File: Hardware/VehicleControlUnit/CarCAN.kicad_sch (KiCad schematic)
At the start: 9 parts, among them IC2 TCAN3413DR

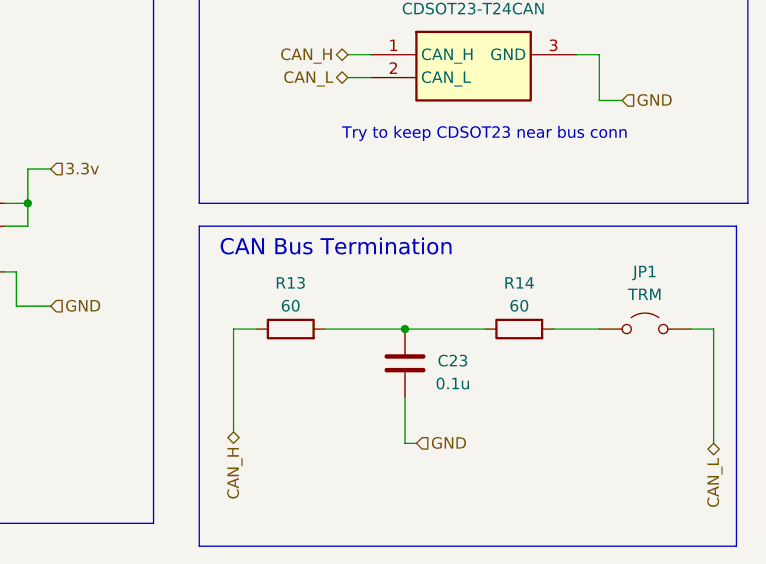
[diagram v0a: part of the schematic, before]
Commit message: 70% tracing done
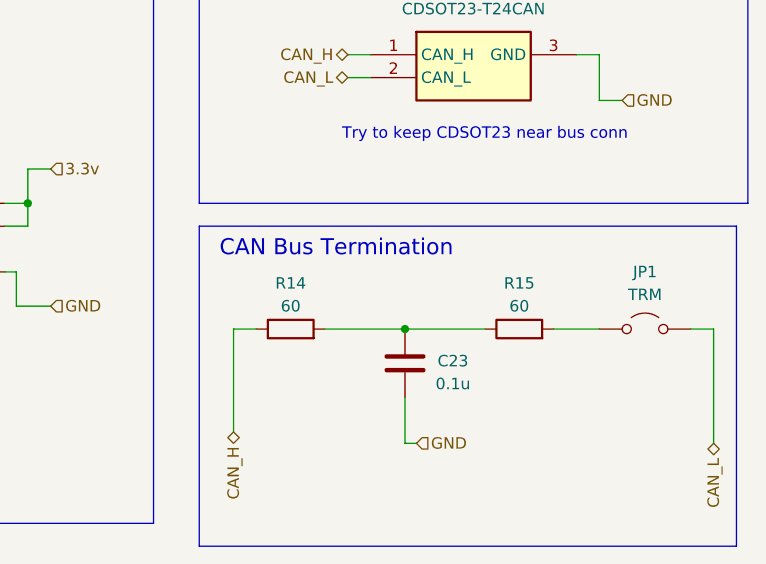
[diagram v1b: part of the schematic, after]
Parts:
- renumbered R13 to R14, R14 to R15
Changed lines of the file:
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@@
 		(in_pos_files yes)
 		(dnp no)
-		(property "Reference" "R14"
+		(property "Reference" "R15"
 			(at 201.93 80.01 90)
 			(show_name no)
@@
 			(project "VehicleControlUnit"
 				(path "/e864fac9-3897-46c9-9101-6d5488c6cd3a/252635d1-b56c-4964-8f6e-39efe20521e2"
-					(reference "R14")
+					(reference "R15")
 					(unit 1)
 				)
@@
 		(in_pos_files yes)
 		(dnp no)
-		(property "Reference" "R13"
+		(property "Reference" "R14"
 			(at 176.53 80.01 90)
 			(show_name no)
@@
 			(project "VehicleControlUnit"
 				(path "/e864fac9-3897-46c9-9101-6d5488c6cd3a/252635d1-b56c-4964-8f6e-39efe20521e2"
-					(reference "R13")
-					(unit 1)
-				)
+					(reference "R14")
+					(unit 1)
+				)

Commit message: i hate this moco, its so stupid why are we doign this.
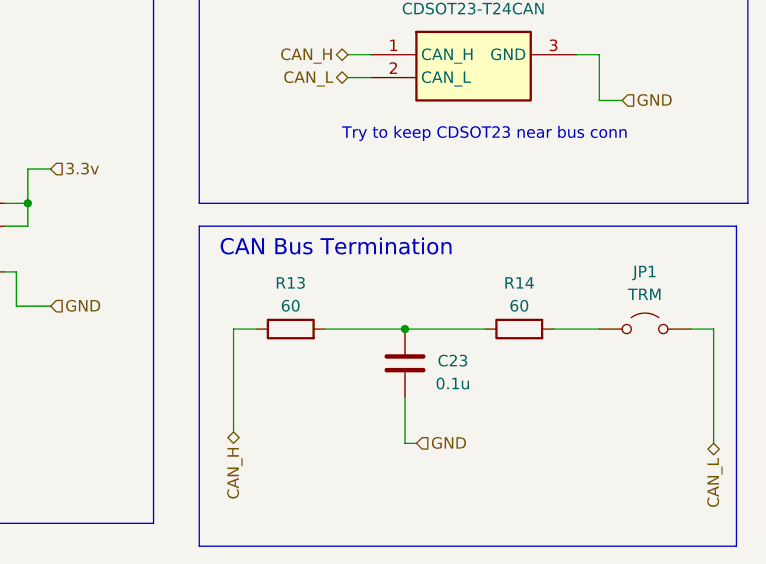
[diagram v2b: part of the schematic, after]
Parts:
- renumbered R14 to R13, R15 to R14
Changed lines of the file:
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@@
 		(in_pos_files yes)
 		(dnp no)
-		(property "Reference" "R15"
+		(property "Reference" "R14"
 			(at 201.93 80.01 90)
 			(show_name no)
@@
 			(project "VehicleControlUnit"
 				(path "/e864fac9-3897-46c9-9101-6d5488c6cd3a/252635d1-b56c-4964-8f6e-39efe20521e2"
-					(reference "R15")
+					(reference "R14")
 					(unit 1)
 				)
@@
 		(in_pos_files yes)
 		(dnp no)
-		(property "Reference" "R14"
+		(property "Reference" "R13"
 			(at 176.53 80.01 90)
 			(show_name no)
@@
 			(project "VehicleControlUnit"
 				(path "/e864fac9-3897-46c9-9101-6d5488c6cd3a/252635d1-b56c-4964-8f6e-39efe20521e2"
-					(reference "R14")
-					(unit 1)
-				)
+					(reference "R13")
+					(unit 1)
+				)
